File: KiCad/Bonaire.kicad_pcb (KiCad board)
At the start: 2 copper layers, 99.5 x 91.2 mm, 77 parts, among them CON1 AVR-JTAG-10, J1 Conn_01x04, J2 Conn_01x04, J3 Conn_01x04, J4 Conn_01x04, J5 Conn_01x04, J6 Conn_01x04, J7 Conn_02x10_Counter_Clockwise, J8 Conn_01x06, Q1 Q_NMOS_GDS, SW1 SW_DPDT_x2, SW2 SW_DPDT_x2, U1 LM78l33_TO220, U2 STM32F303V(B-C)Tx_u, U3 SN65HV7X, U4 MAX31865, U5 MAX31865, U6 MAX31865, U7 MAX31865, U8 MAX31865

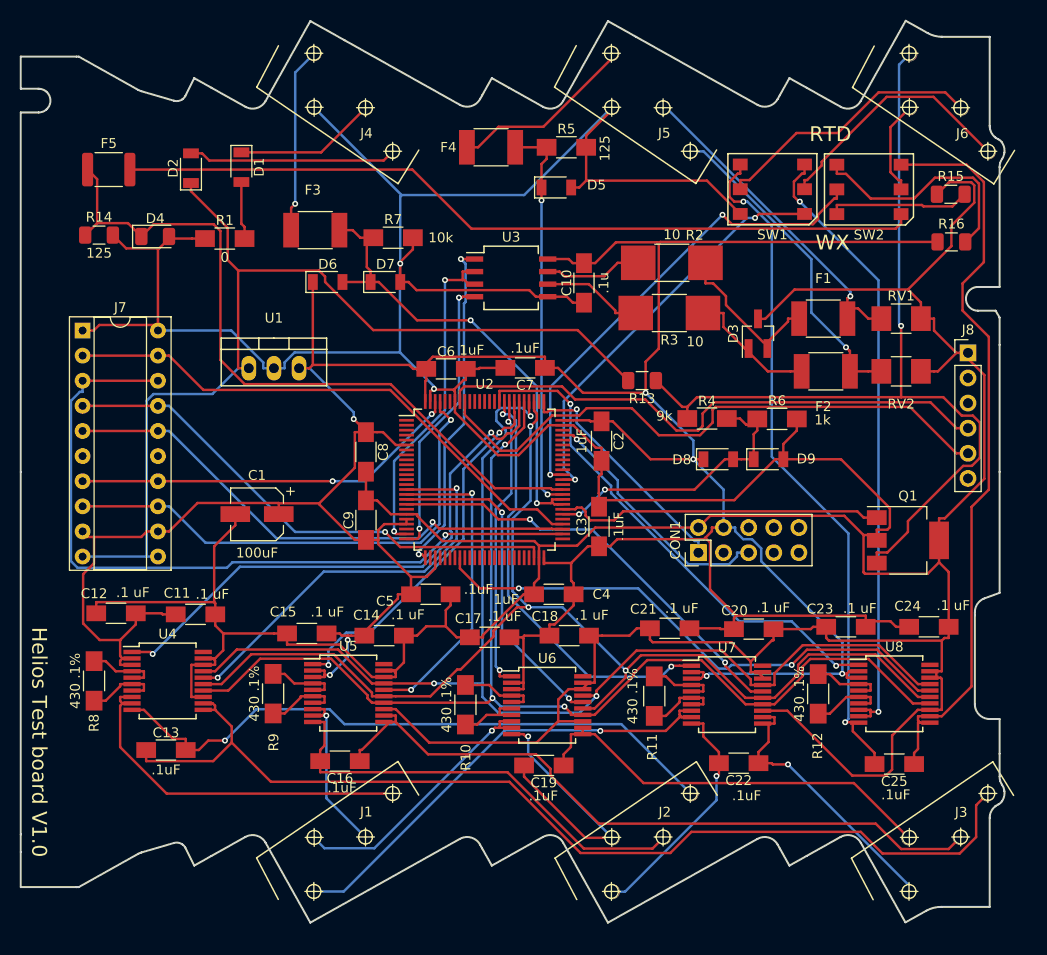
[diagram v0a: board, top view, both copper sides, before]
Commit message: Have board layout done, need to route
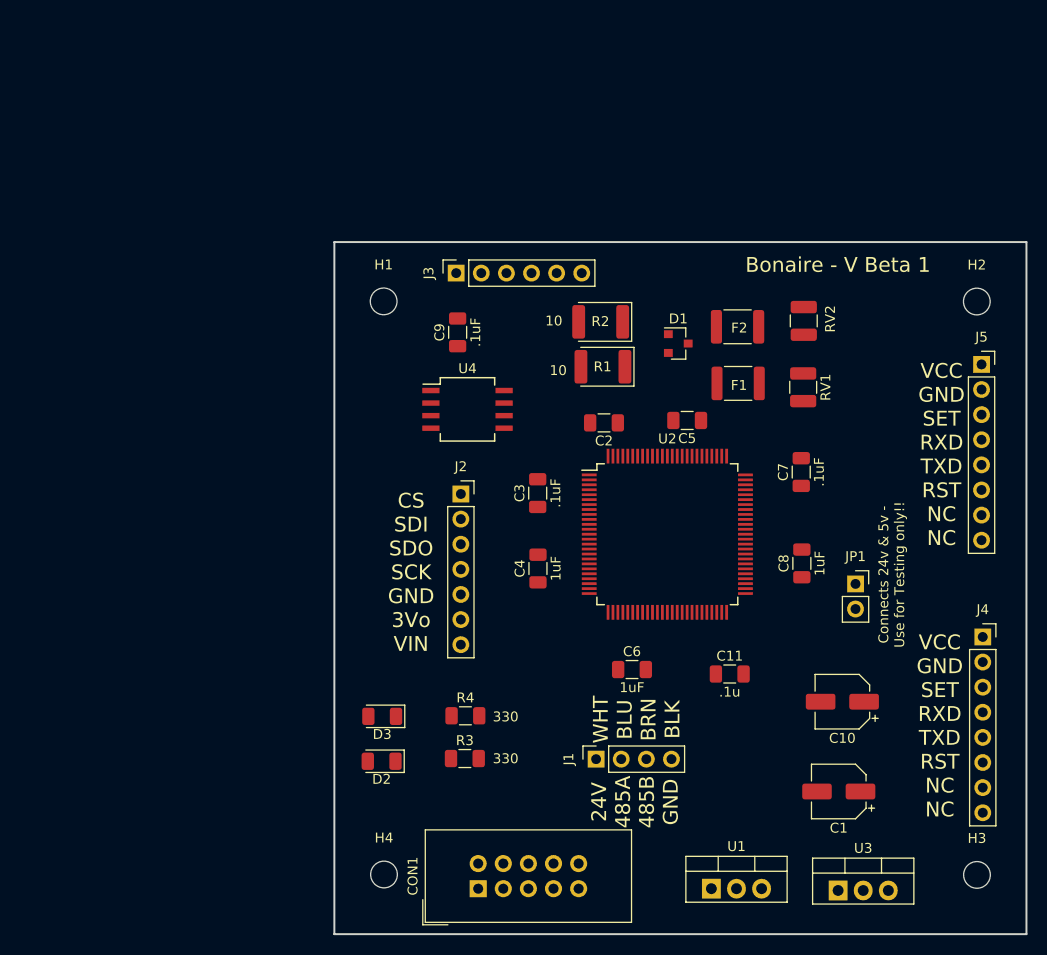
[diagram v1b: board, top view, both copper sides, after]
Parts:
- removed C12, C14, C15, C17, C18, C20, C21, C23, C24: .1 uF, Capacitors_SMD:C_1206_HandSoldering
- removed C13, C16, C19, C22, C25: .1uF, Capacitors_SMD:C_1206_HandSoldering
- removed D4: D_Schottky, Diode_SMD:D_1206_3216Metric
- removed D5, D6, D7, D8, D9: D_Schottky, Diodes_SMD:D_1206
- removed F3, F4: Polyfuse_Small, Resistors_SMD:R_1812
- removed F5: Polyfuse_Small, Resistor_SMD:R_1812_4532Metric
- removed J6: Conn_01x04, CH20M:CH20Mt
- removed J7: Conn_02x10_Counter_Clockwise, Package_DIP:DIP-20_W7.62mm_Socket
- removed J8: Conn_01x06, Pin_Headers:Pin_Header_Straight_1x06_Pitch2.54mm
- removed Q1: Q_NMOS_GDS, Package_TO_SOT_SMD:SOT-223-3_TabPin2
- removed R10, R11, R12, R8, R9: 430 .1%, Resistors_SMD:R_1206_HandSoldering
- removed R13, R15, R16: 10k, Resistor_SMD:R_1206_3216Metric
- removed R14: 125, Resistor_SMD:R_1206_3216Metric
- removed R5: 125, Resistors_SMD:R_1206_HandSoldering
- removed R6: 1k, Resistors_SMD:R_1206_HandSoldering
- removed R7: 10k, Resistors_SMD:R_1206_HandSoldering
- removed SW1, SW2: SW_DPDT_x2, CH20M:DPDT
- removed U5, U6, U7, U8: MAX31865, Housings_SSOP:SSOP-20_5.3x7.2mm_Pitch0.65mm
- added H1: MountingHole, MountingHole:MountingHole_2.7mm_M2.5, F.Cu at (125.8, 72.0)
- added H2: MountingHole, MountingHole:MountingHole_2.7mm_M2.5, F.Cu at (185.8, 72.0)
- added H3: MountingHole, MountingHole:MountingHole_2.7mm_M2.5, F.Cu at (185.8, 130.0)
- added H4: MountingHole, MountingHole:MountingHole_2.7mm_M2.5, F.Cu at (125.8, 129.9)
- added JP1: Jumper, Connector_PinSocket_2.54mm:PinSocket_1x02_P2.54mm_Vertical, F.Cu at (173.5, 100.5)
- C1: footprint Capacitors_SMD:CP_Elec_5x5.3 -> Capacitor_SMD:CP_Elec_5x5.3
- C10: value .1u -> 100uF; footprint Capacitors_SMD:C_1206_HandSoldering -> Capacitor_SMD:CP_Elec_5x5.3
- C11: value .1 uF -> .1u; footprint Capacitors_SMD:C_1206_HandSoldering -> Capacitor_SMD:C_1206_3216Metric
- C2, C3, C4, C5, C6, C7, C8, C9: footprint Capacitors_SMD:C_1206_HandSoldering -> Capacitor_SMD:C_1206_3216Metric
- CON1: footprint Pin_Headers:Pin_Header_Straight_2x05_Pitch2.54mm -> Connector_IDC:IDC-Header_2x05_P2.54mm_Vertical
- D1: value D_Schottky -> D_TVS_x2_AAC; footprint Diodes_SMD:D_1206 -> Package_TO_SOT_SMD:SOT-23
- D2: value D_Schottky -> LED; footprint Diodes_SMD:D_1206 -> LED_SMD:LED_1206_3216Metric
- D3: value D_TVS_x2_AAC -> LED; footprint TO_SOT_Packages_SMD:SOT-23_Handsoldering -> LED_SMD:LED_1206_3216Metric
- F1, F2: footprint Resistors_SMD:R_1812 -> Resistor_SMD:R_1812_4532Metric
- J1: footprint CH20M:CH20Mr -> Connector_PinSocket_2.54mm:PinSocket_1x04_P2.54mm_Vertical
- J2: value Conn_01x04 -> Conn_01x07; footprint CH20M:CH20Mr -> Connector_PinSocket_2.54mm:PinSocket_1x07_P2.54mm_Vertical
- J3: value Conn_01x04 -> Conn_01x06; footprint CH20M:CH20Mr -> Connector_PinSocket_2.54mm:PinSocket_1x06_P2.54mm_Vertical
- J4, J5: value Conn_01x04 -> Conn_01x08; footprint CH20M:CH20Mt -> Connector_PinSocket_2.54mm:PinSocket_1x08_P2.54mm_Vertical
- R1: value 0 -> 10; footprint Resistors_SMD:R_1206_HandSoldering -> Diode_SMD:D_1812_4532Metric_Pad1.30x3.40mm_HandSolder
- R2: footprint Resistors_SMD:R_1812_HandSoldering -> Diode_SMD:D_1812_4532Metric_Pad1.30x3.40mm_HandSolder
- R3: value 10 -> 330; footprint Resistors_SMD:R_1812_HandSoldering -> Resistor_SMD:R_1206_3216Metric
- R4: value 9k -> 330; footprint Resistors_SMD:R_1206_HandSoldering -> Resistor_SMD:R_1206_3216Metric
- RV1, RV2: footprint Resistors_SMD:R_1210_HandSoldering -> Resistor_SMD:R_1210_3225Metric
- U1: footprint TO_SOT_Packages_THT:TO-220_Neutral123_Vertical -> Package_TO_SOT_THT:TO-220-3_Vertical
- U2: footprint Housings_QFP:LQFP-100_14x14mm_Pitch0.5mm -> Package_QFP:LQFP-100_14x14mm_P0.5mm
- U3: value SN65HV7X -> LM78l50_TO220; footprint Housings_SOIC:SO-8_5.3x6.2mm_Pitch1.27mm -> Package_TO_SOT_THT:TO-220-3_Vertical
- U4: value MAX31865 -> SN65HV7X; footprint Housings_SSOP:SSOP-20_5.3x7.2mm_Pitch0.65mm -> Package_SO:SO-8_5.3x6.2mm_P1.27mm
- moved J4 84.1 mm to (186.4, 105.9)
- moved J3 75.7 mm to (133.1, 69.1), turned to 90 degrees
- moved U3 70.2 mm to (171.8, 131.6)
- moved U1 68.8 mm to (158.9, 131.4)
- moved C1 65.2 mm to (171.8, 121.5)
- moved D2 63.0 mm to (125.6, 118.5), turned to 180 degrees
- moved C11 54.4 mm to (160.8, 109.7), turned to 0 degrees
- moved D3 54.2 mm to (125.6, 113.9), turned to 180 degrees
- moved C10 49.8 mm to (172.2, 112.5), turned to 180 degrees
- moved R3 49.6 mm to (134.0, 118.2), turned to 0 degrees
- moved D1 47.7 mm to (155.6, 76.2), turned to 0 degrees
- moved C8 45.5 mm to (168.1, 98.5), turned to 90 degrees
- moved J5 43.2 mm to (186.3, 78.3)
- moved U4 40.9 mm to (134.3, 82.9)
- moved CON1 40.6 mm to (135.4, 131.4)
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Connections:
- C10 pad 1: GND -> +5V
- C10 pad 2: +3V3 -> GND
- D1 pad 1: GNDPWR -> Net-(D1-Pad1)
- D2 pad 1: +24V -> Net-(D2-Pad1)
- F1 pad 2: Net-(D3-Pad2) -> Net-(D1-Pad2)
- F2 pad 2: Net-(D3-Pad1) -> Net-(D1-Pad1)
- J1 pad 1: RTDa1 -> +24V
- J1 pad 2: RTDa2 -> /RS485A
- J1 pad 3: RTDa3 -> /RS485B
- J1 pad 4: RTDa4 -> GND
- J2 pad 1: RTDb1 -> /GPIOB/~CS
- J2 pad 2: RTDb2 -> /GPIOB/MOSI
- J2 pad 3: RTDb3 -> /GPIOB/MISO
- J2 pad 4: RTDb4 -> /GPIOB/SCK
- J3 pad 1: RTD-1 -> GND
- J3 pad 2: RTD-2 -> Net-(J3-Pad2)
- J3 pad 3: RTD-3 -> +5V
- J3 pad 4: RTD-4 -> /GPIOB/UART1_RX
- J4 pad 1: Net-(D2-Pad2) -> GND
- J4 pad 2: GNDPWR -> +5V
- J4 pad 3: GND -> Net-(J4-Pad3)
- J4 pad 4: /Pyro -> Net-(J4-Pad4)
- J5 pad 1: /RS485A -> GND
- J5 pad 2: /RS485B -> +5V
- J5 pad 3: GND -> Net-(J5-Pad3)
- J5 pad 4: /Wind -> Net-(J5-Pad4)
- R1 pad 1: GND -> Net-(D1-Pad2)
- R1 pad 2: Net-(D1-Pad2) -> Net-(R1-Pad2)
- R2 pad 1: Net-(D3-Pad2) -> Net-(D1-Pad1)
- R3 pad 1: Net-(D3-Pad1) -> Net-(D2-Pad1)
- R3 pad 2: Net-(R3-Pad2) -> GND
- R4 pad 1: Net-(D8-Pad2) -> Net-(D3-Pad1)
- R4 pad 2: /Snow -> GND
- U2 pad 15: ~RTDcs1 -> Net-(U2-Pad15)
- U2 pad 16: ~RTDcs2 -> Net-(U2-Pad16)
- U2 pad 17: ~RTDcs3 -> Net-(U2-Pad17)
- U2 pad 18: ~RTDcs4 -> Net-(U2-Pad18)
- U2 pad 33: ~RTDcs5 -> Net-(U2-Pad33)
- U2 pad 53: /GPIOB/D/~C -> /GPIOB/MISO
- U2 pad 55: Net-(U2-Pad55) -> Net-(J5-Pad4)
- U2 pad 56: Net-(D8-Pad2) -> Net-(J5-Pad5)
- U2 pad 57: Net-(Q1-Pad1) -> Net-(J5-Pad6)
- U2 pad 58: Net-(D6-Pad2) -> Net-(U2-Pad58)
- U2 pad 59: Net-(D6-Pad2) -> Net-(U2-Pad59)
- U2 pad 63: Rain -> Net-(U2-Pad63)
- U2 pad 64: Aux -> Net-(U2-Pad64)
- U2 pad 66: Net-(U2-Pad66) -> Net-(J4-Pad3)
- U2 pad 78: RTD_SCK -> Net-(J4-Pad4)
- U2 pad 79: RTD_MISO -> Net-(J4-Pad5)
- U2 pad 80: RTD_MOSI -> Net-(J4-Pad6)
- U2 pad 81: ~DRDY1 -> Net-(U2-Pad81)
- U2 pad 82: ~DRDY2 -> Net-(U2-Pad82)
- U2 pad 83: ~DRDY3 -> Net-(U2-Pad83)
- U2 pad 84: ~DRDY4 -> Net-(U2-Pad84)
- U2 pad 85: ~DRDY5 -> Net-(U2-Pad85)
- U2 pad 88: Net-(U2-Pad88) -> Net-(J5-Pad3)
- U2 pad 97: /GPIOB/485RX -> Net-(D3-Pad2)
- U2 pad 98: /GPIOB/485TX -> Net-(D2-Pad2)
- U3 pad 1: /GPIOA/serial/RX -> +24V
- U3 pad 2: /GPIOA/serial/TX_en -> GND
- U3 pad 3: /GPIOA/serial/TX_en -> +5V
- U4 pad 1: ~DRDY1 -> /GPIOA/serial/RX
- U4 pad 2: +3V3 -> /GPIOA/serial/TX_en
- U4 pad 3: +3V3 -> /GPIOA/serial/TX_en
- U4 pad 4: Net-(R8-Pad1) -> /GPIOA/serial/TX
- U4 pad 5: Net-(R8-Pad1) -> GND
- U4 pad 6: Net-(R8-Pad2) -> Net-(R2-Pad2)
- U4 pad 7: Net-(R8-Pad2) -> Net-(R1-Pad2)
- U4 pad 8: RTDa1 -> +3V3
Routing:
- net GND: track 599.1 -> 0.00 mm, vias 2 -> 0
- net +3V3: track 374.8 -> 0.00 mm, vias 7 -> 0
- net RTD_MISO: track 122.3 -> 0.00 mm, vias 3 -> 0
- net RTD_SCK: track 119.0 -> 0.00 mm, vias 3 -> 0
- net RTD_MOSI: track 118.0 -> 0.00 mm, vias 3 -> 0
- net RTD-1: track 104.7 -> 0.00 mm
- net +24V: track 101.2 -> 0.00 mm
- net /Snow: track 91.5 -> 0.00 mm, vias 1 -> 0
- net WindDir: track 81.6 -> 0.00 mm
- net /GPIOB/SCK: track 78.1 -> 0.00 mm, vias 1 -> 0
- net RTD-5: track 75.8 -> 0.00 mm
- net Net-(U2-Pad61): track 74.4 -> 0.00 mm
- net RTD-2: track 71.7 -> 0.00 mm
- net RTDb5: track 69.4 -> 0.00 mm, vias 2 -> 0
- net RTDb1: track 64.1 -> 0.00 mm, vias 1 -> 0
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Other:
- board size 99.5 x 91.2 mm -> 70 x 70 mm
- board text added: "24V 485A 485B GND"
- board text added: "Bonaire - V Beta 1"
- board text added: "CS SDI SDO SCK GND 3Vo VIN"
- board text added: "Connects 24v & 5v - Use for Testing only!!"
- board text added: "VCC GND SET RXD TXD RST NC NC"
- board text added: "WHT BLU BRN BLK"
- board text removed: "Helios Test board V1.0"
- board text removed: "RTD"
- board text removed: "WX"
